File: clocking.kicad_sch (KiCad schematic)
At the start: 0 parts

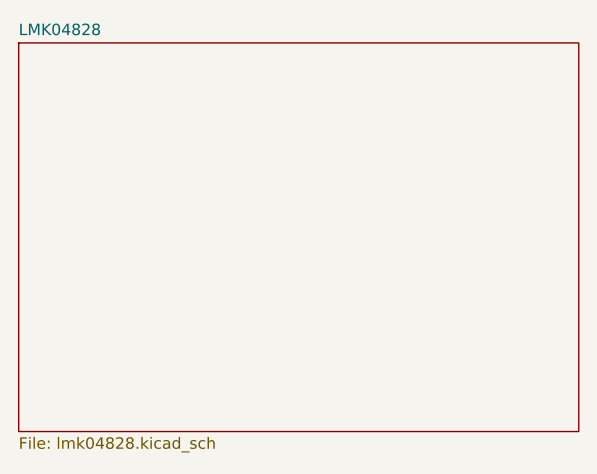
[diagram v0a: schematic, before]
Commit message: Complete LMK schematic
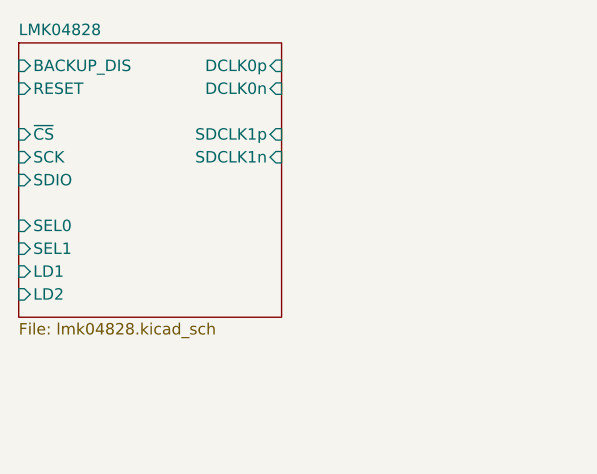
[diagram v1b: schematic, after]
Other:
- sheet LMK04828 ports: added BACKUP_DIS, DCLK0n, DCLK0p, LD1, LD2, RESET, SCK, SDCLK1n, SDCLK1p, SDIO, SEL0, SEL1, ~{CS}; removed none
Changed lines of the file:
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@@
 	(sheet
 		(at 54.61 50.8)
-		(size 62.23 43.18)
+		(size 29.21 30.48)
 		(exclude_from_sim no)
 		(in_bom yes)
@@
 		)
 		(property "Sheetfile" "lmk04828.kicad_sch"
-			(at 54.61 94.5646 0)
+			(at 54.61 81.8646 0)
 			(effects
 				(font
@@
 			)
 		)
+		(pin "BACKUP_DIS" input
+			(at 54.61 53.34 180)
+			(effects
+				(font
+					(size 1.27 1.27)
+				)
+				(justify left)
+			)
+		)
+		(pin "DCLK0n" input
+			(at 83.82 55.88 0)
+			(effects
+				(font
+					(size 1.27 1.27)
+				)
+				(justify right)
+			)
+		)
+		(pin "DCLK0p" input
+			(at 83.82 53.34 0)
+			(effects
+				(font
+					(size 1.27 1.27)
+				)
+				(justify right)
+			)
+		)
+		(pin "LD1" input
+			(at 54.61 76.2 180)
+			(effects
+				(font
+					(size 1.27 1.27)
+				)
+				(justify left)
+			)
+		)
+		(pin "LD2" input
+			(at 54.61 78.74 180)
+			(effects
+				(font
+					(size 1.27 1.27)
+				)
+				(justify left)
+			)
+		)
+		(pin "RESET" input
+			(at 54.61 55.88 180)
+			(effects
+				(font
+					(size 1.27 1.27)
+				)
+				(justify left)
+			)
+		)
+		(pin "SCK" input
+			(at 54.61 63.5 180)
+			(effects
+				(font
+					(size 1.27 1.27)
+				)
+				(justify left)
+			)
+		)
+		(pin "SDCLK1n" input
+			(at 83.82 63.5 0)
+			(effects
+				(font
+					(size 1.27 1.27)
+				)
+				(justify right)
+			)
+		)
+		(pin "SDCLK1p" input
+			(at 83.82 60.96 0)
+			(effects
+				(font
+					(size 1.27 1.27)
+				)
+				(justify right)
+			)
+		)
+		(pin "SDIO" input
+			(at 54.61 66.04 180)
+			(effects
+				(font
+					(size 1.27 1.27)
+				)
+				(justify left)
+			)
+		)
+		(pin "SEL0" input
+			(at 54.61 71.12 180)
+			(effects
+				(font
+					(size 1.27 1.27)
+				)
+				(justify left)
+			)
+		)
+		(pin "SEL1" input
+			(at 54.61 73.66 180)
+			(effects
+				(font
+					(size 1.27 1.27)
+				)
+				(justify left)
+			)
+		)
+		(pin "~{CS}" input
+			(at 54.61 60.96 180)
+			(effects
+				(font
+					(size 1.27 1.27)
+				)
+				(justify left)
+			)
+		)

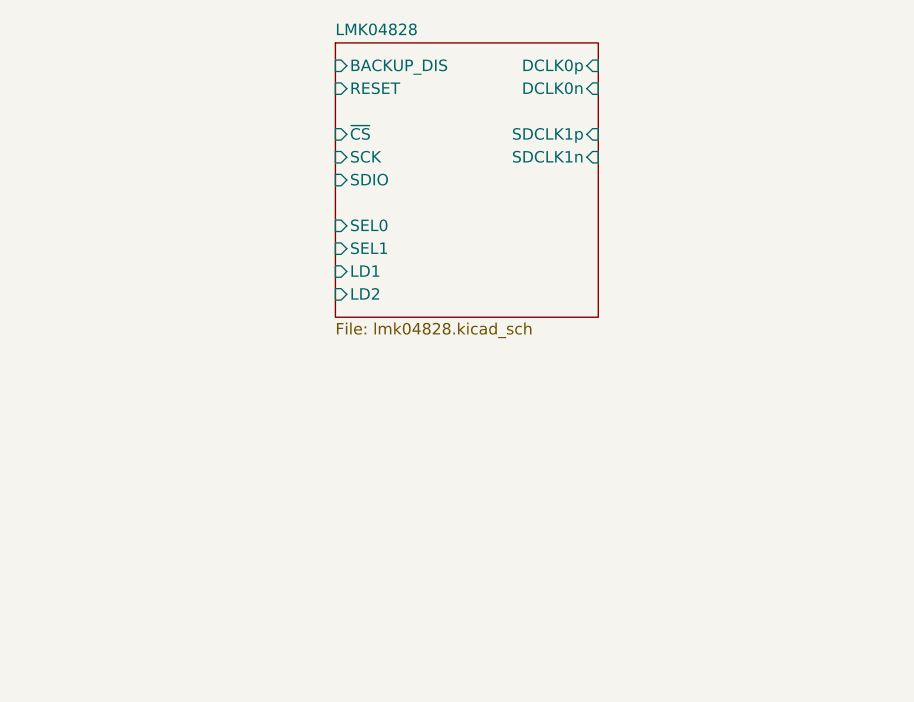
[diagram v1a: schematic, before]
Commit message: Add LMX Draft
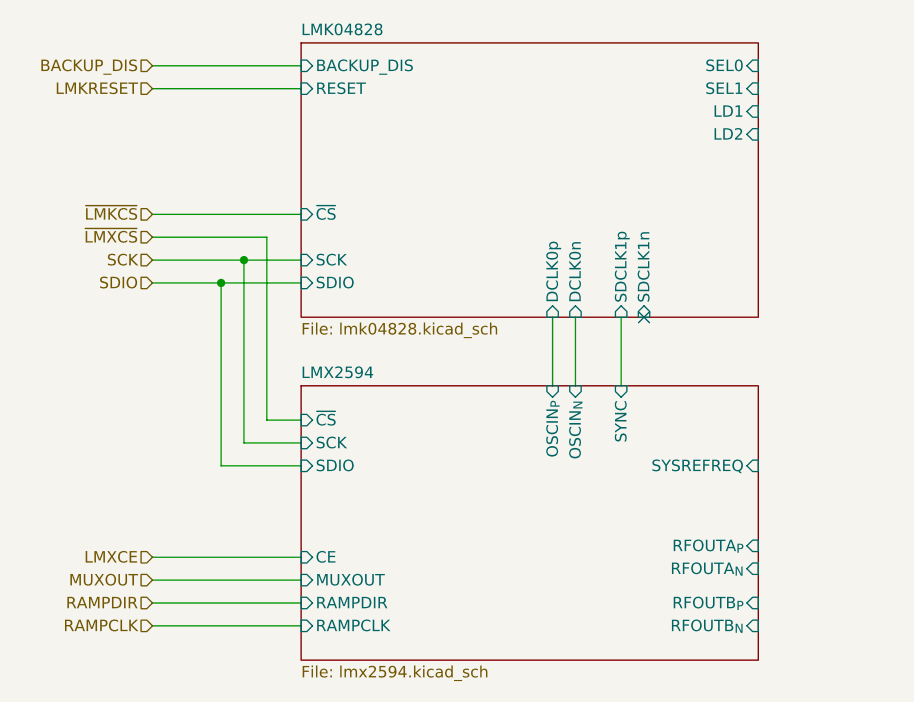
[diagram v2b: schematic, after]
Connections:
- no-connect marks 0 -> 1
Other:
- added sheet LMX2594 (lmx2594.kicad_sch)
